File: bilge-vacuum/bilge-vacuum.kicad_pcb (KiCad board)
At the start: 4 copper layers, 163 x 133 mm, 194 parts, among them J1 TC2030-SWD, J2 Screw_Terminal_01x02, J3 Screw_Terminal_01x02, J4 Screw_Terminal_01x02, J5 Screw_Terminal_01x02, J6 Screw_Terminal_01x02, J7 Screw_Terminal_01x02, J8 Screw_Terminal_01x02, Q1 PSMN014-80YL, Q10 Q_NMOS_GSD, Q11 PSMN014-80YL, Q2 PSMN014-80YL, Q3 PSMN014-80YL, Q4 PSMN014-80YL, Q5 PMV65XP,215, Q6 PSMN014-80YL, Q7 Q_NMOS_GSD, Q8 Q_PMOS_GSD, Q9 Q_PMOS_GSD, SW1 B3F-1000, U1 STM32G0B1CEU6, U10 TPS27S100A, U11 TPS27S100A, U12 NHD-C12864A1Z-FSW-FBW-HTT, U13 ADP151, U14 FM25V20A, U2 LTC3851, U3 LTC3786, U4 MAX14626, U5 LTC4229, U6 LMV321, U7 TPS27S100A, U8 TPS27S100A, U9 TPS27S100A

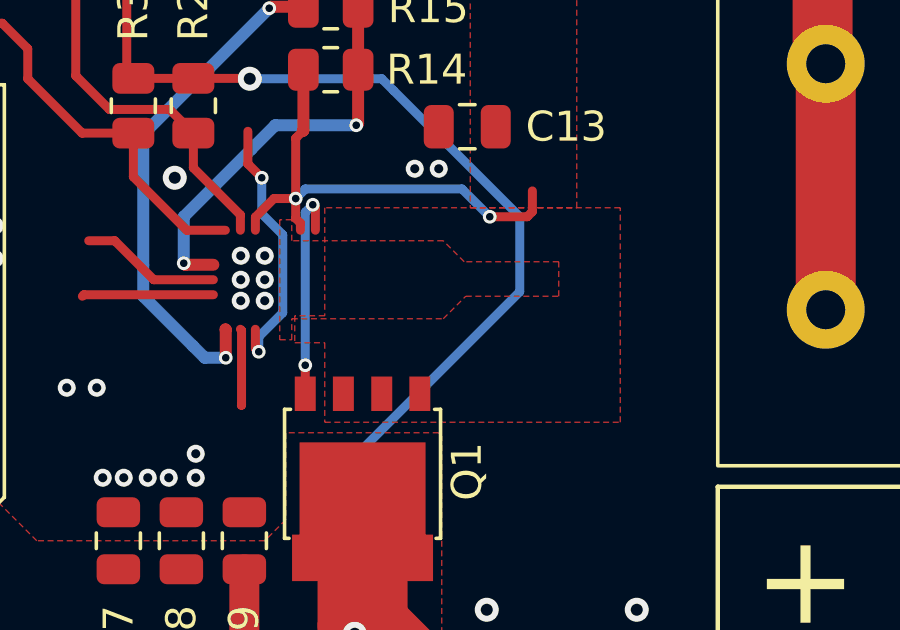
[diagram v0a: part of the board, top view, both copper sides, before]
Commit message: E Paper Hum WIP
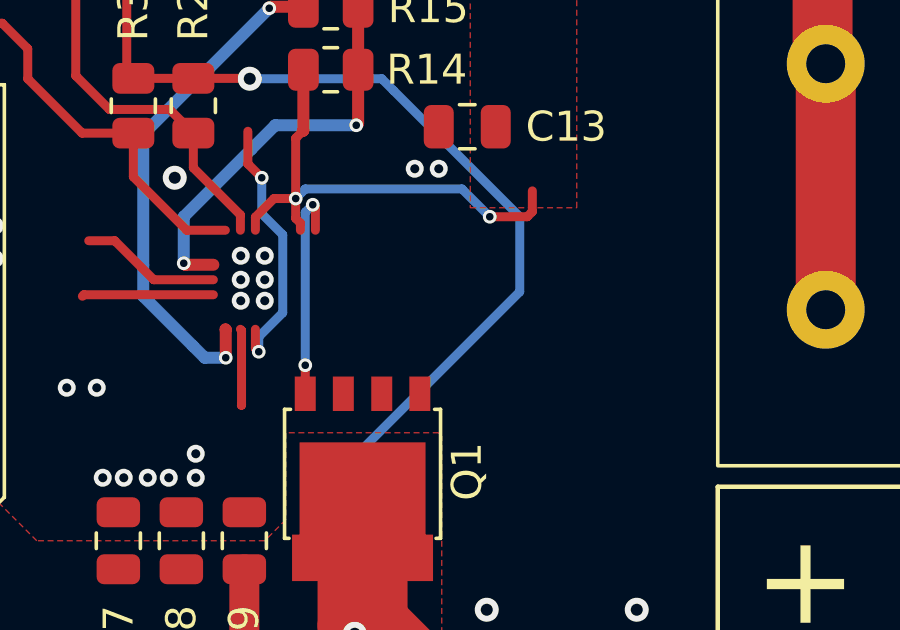
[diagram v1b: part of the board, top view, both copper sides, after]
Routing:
- removed copper zone on F.Cu, net (none)
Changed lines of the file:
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@@
-    )
-  )
-  (zone (net 7) (net_name "+12V") (layer "F.Cu") (hatch edge 0.5)
-    (priority 16)
-    (connect_pads yes (clearance 0.127))
-    (min_thickness 0.127) (filled_areas_thickness no)
-    (fill yes (thermal_gap 0.4) (thermal_bridge_width 1))
-    (polygon
-      (pts
-        (xy 110.6 135.9)
-        (xy 110.6 139.5)
-        (xy 109.6 139.5)
-        (xy 109.6 140.4)
-        (xy 110.6 140.4)
-        (xy 110.6 143.05)
-        (xy 120.45 143.05)
-        (xy 120.45 135.9)
-      )
     )
   )
@@
       )
     )
-  )
-  (zone (net 0) (net_name "") (layer "F.Cu") (hatch edge 0.5)
-    (priority 17)
-    (connect_pads yes (clearance 0.254))
-    (min_thickness 0.25) (filled_areas_thickness no)
-    (fill yes (thermal_gap 0.4) (thermal_bridge_width 1))
-    (polygon
-      (pts
-        (xy 118.4 137.7)
-        (xy 115.25 137.7)
-        (xy 114.55 137)
-        (xy 109.5 137)
-        (xy 109.5 136.3)
-        (xy 109.1 136.3)
-        (xy 109.1 140.3)
-        (xy 109.5 140.3)
-        (xy 109.5 139.6)
-        (xy 114.55 139.6)
-        (xy 115.3 138.85)
-        (xy 118.4 138.85)
-      )
-    )
